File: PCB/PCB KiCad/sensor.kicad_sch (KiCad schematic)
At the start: 12 parts, among them U1 OPA2376AID

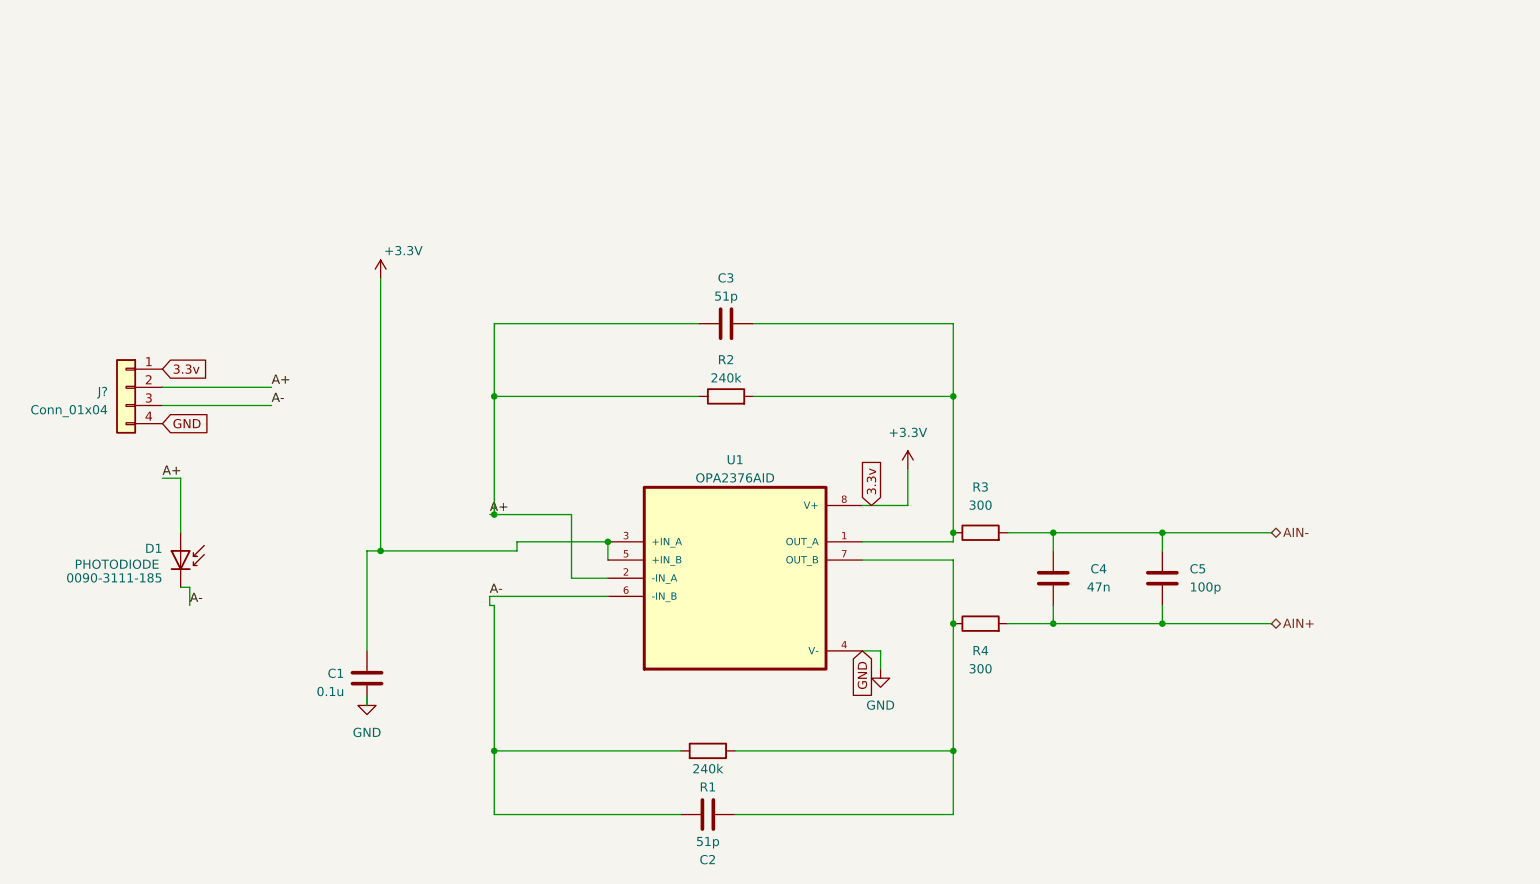
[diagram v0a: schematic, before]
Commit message: Minor schematic cleanup!
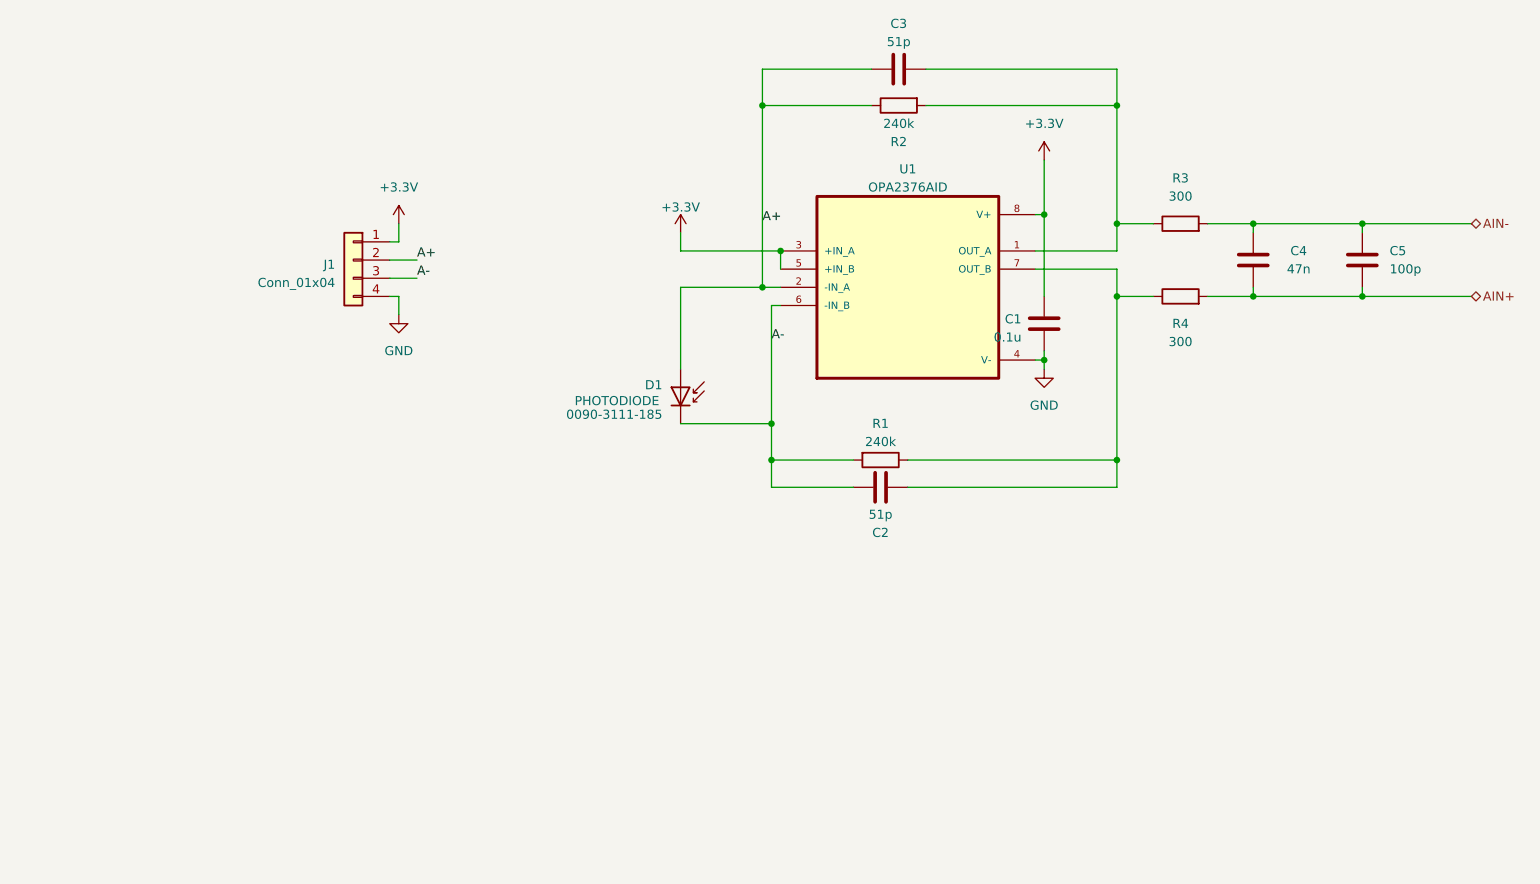
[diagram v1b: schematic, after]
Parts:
- D1: footprint Diode_THT:D_A-405_P2.54mm_Vertical_KathodeUp -> Diode_SMD:D_1206_3216Metric_Pad1.42x1.75mm_HandSolder
- gave numbers to parts that had none: 1
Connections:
- net +3V3 renamed +3.3V
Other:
- moved on the sheet: C1, C2, C3, C4, C5, D1, J1, R1, R2, R3, R4, U1
